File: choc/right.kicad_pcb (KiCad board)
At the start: 2 copper layers, 117 x 92 mm, 63 parts, among them J2 USB_B_Micro, SW24 SW_Push, SW25 SW_Push, SW26 SW_Push, SW27 SW_Push, SW28 SW_Push, SW29 SW_Push, SW30 SW_Push, SW31 SW_Push, SW32 SW_Push, SW33 SW_Push, SW34 SW_Push, SW35 SW_Push, SW36 SW_Push, SW37 SW_Push, SW38 SW_Push, SW39 SW_Push, SW40 SW_Push, SW41 SW_Push, SW42 SW_Push, SW43 SW_Push, SW44 SW_Push, SW45 SW_Push, SW46 SW_Push, SW48 SW_Push, SW50 SW_Push, U2 ProMicro

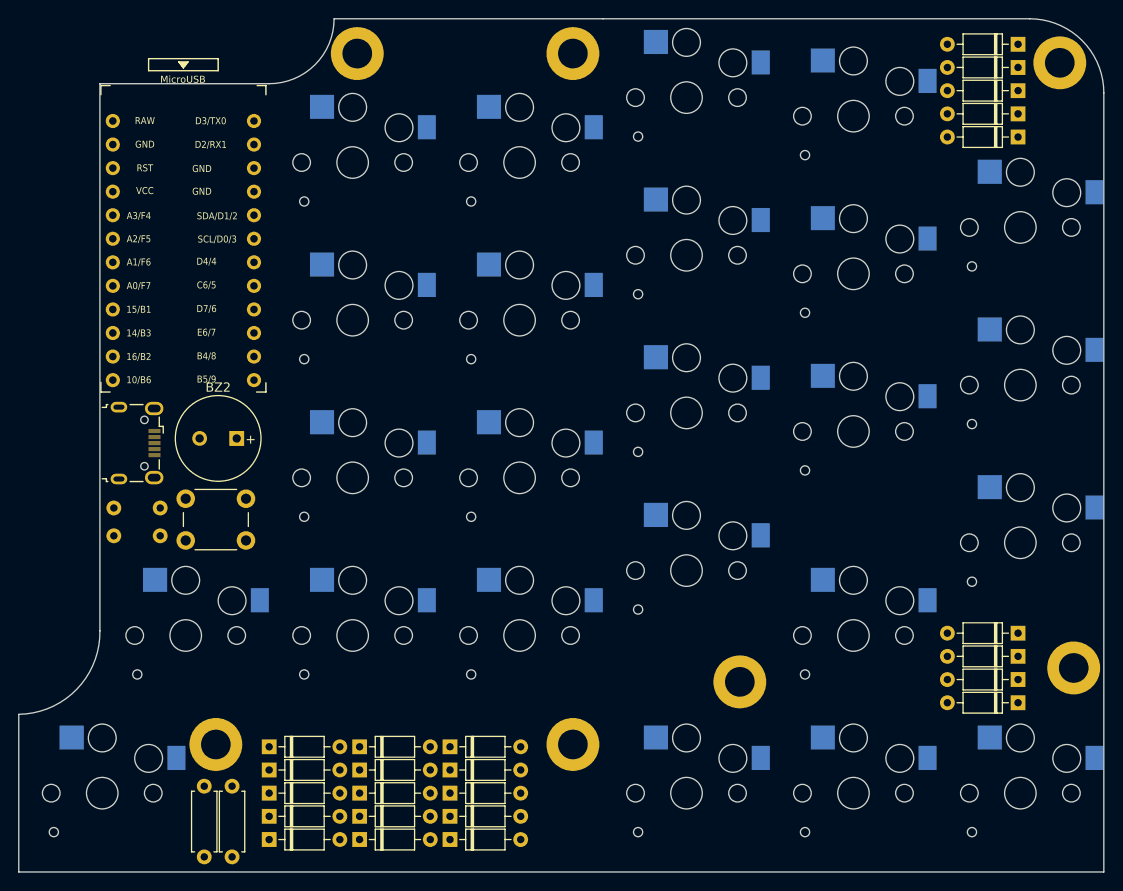
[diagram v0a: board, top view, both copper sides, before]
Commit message: import right ses
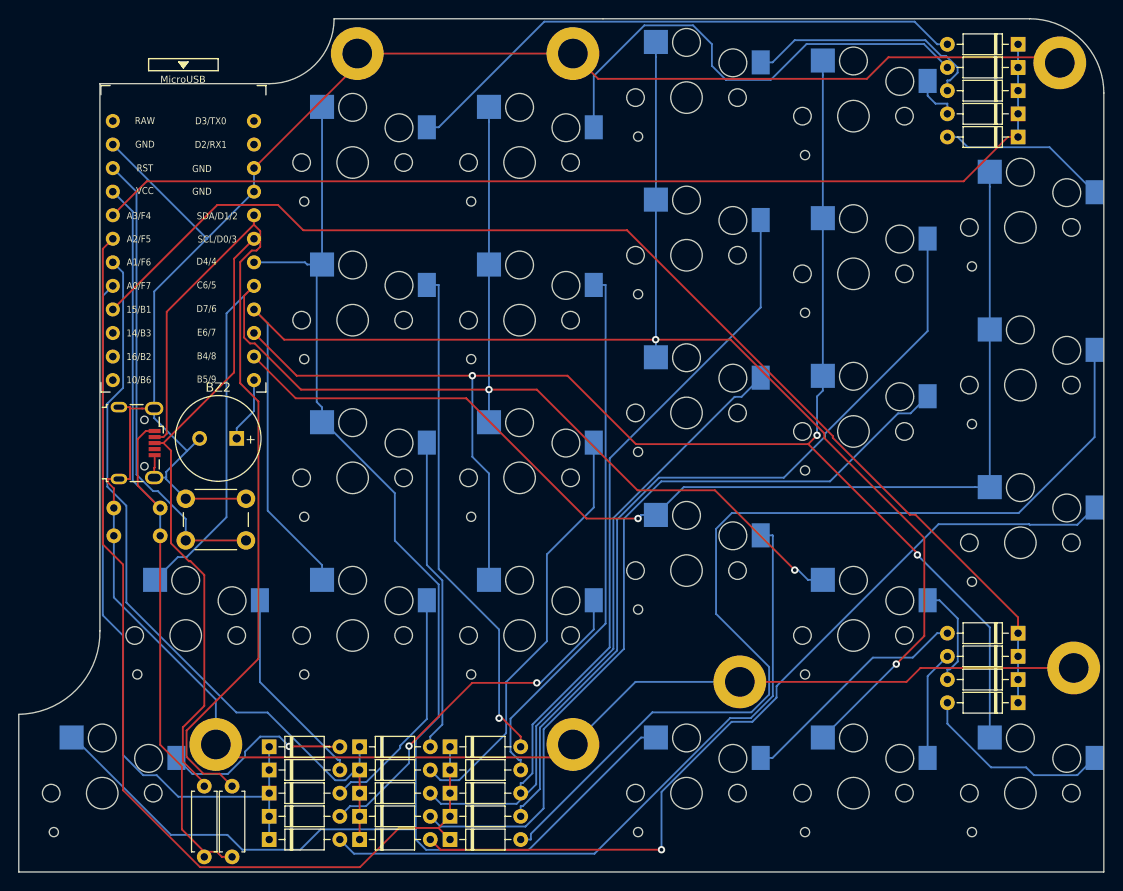
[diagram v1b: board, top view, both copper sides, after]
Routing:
- net GND: track 0.00 -> 309.4 mm
- net /rcol2: track 0.00 -> 175.0 mm, vias 0 -> 2
- net /rcol3: track 0.00 -> 169.2 mm, vias 0 -> 3
- net /rcol0: track 0.00 -> 167.4 mm
- net /rcol1: track 0.00 -> 149.9 mm, vias 0 -> 2
- net /rrow4: track 0.00 -> 130.0 mm
- net /rcol4: track 0.00 -> 122.0 mm, vias 0 -> 1
- net /rrow0: track 0.00 -> 111.1 mm
- net /rrow1: track 0.00 -> 111.0 mm
- net Net-(D44-Pad2): track 0.00 -> 108.2 mm
- net /rSDA: track 0.00 -> 98.0 mm
- net Net-(D45-Pad2): track 0.00 -> 91.8 mm, vias 0 -> 1
- net +5V: track 0.00 -> 89.7 mm
- net Net-(D40-Pad2): track 0.00 -> 88.5 mm
- net Net-(D41-Pad2): track 0.00 -> 86.5 mm
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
